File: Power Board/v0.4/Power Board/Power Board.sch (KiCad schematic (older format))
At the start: 31 parts, among them J1 Battery In, J2 JST B2PS-VH, J3 JST B2PS-VH, J4 JST B2PS-VH, J5 JST B2PS-VH, J6 JST B2PS-VH, J7 JST B2PS-VH, J8 Molex 70553-0006, J9 Conn_02x05_Odd_Even, SW1 SW_Push

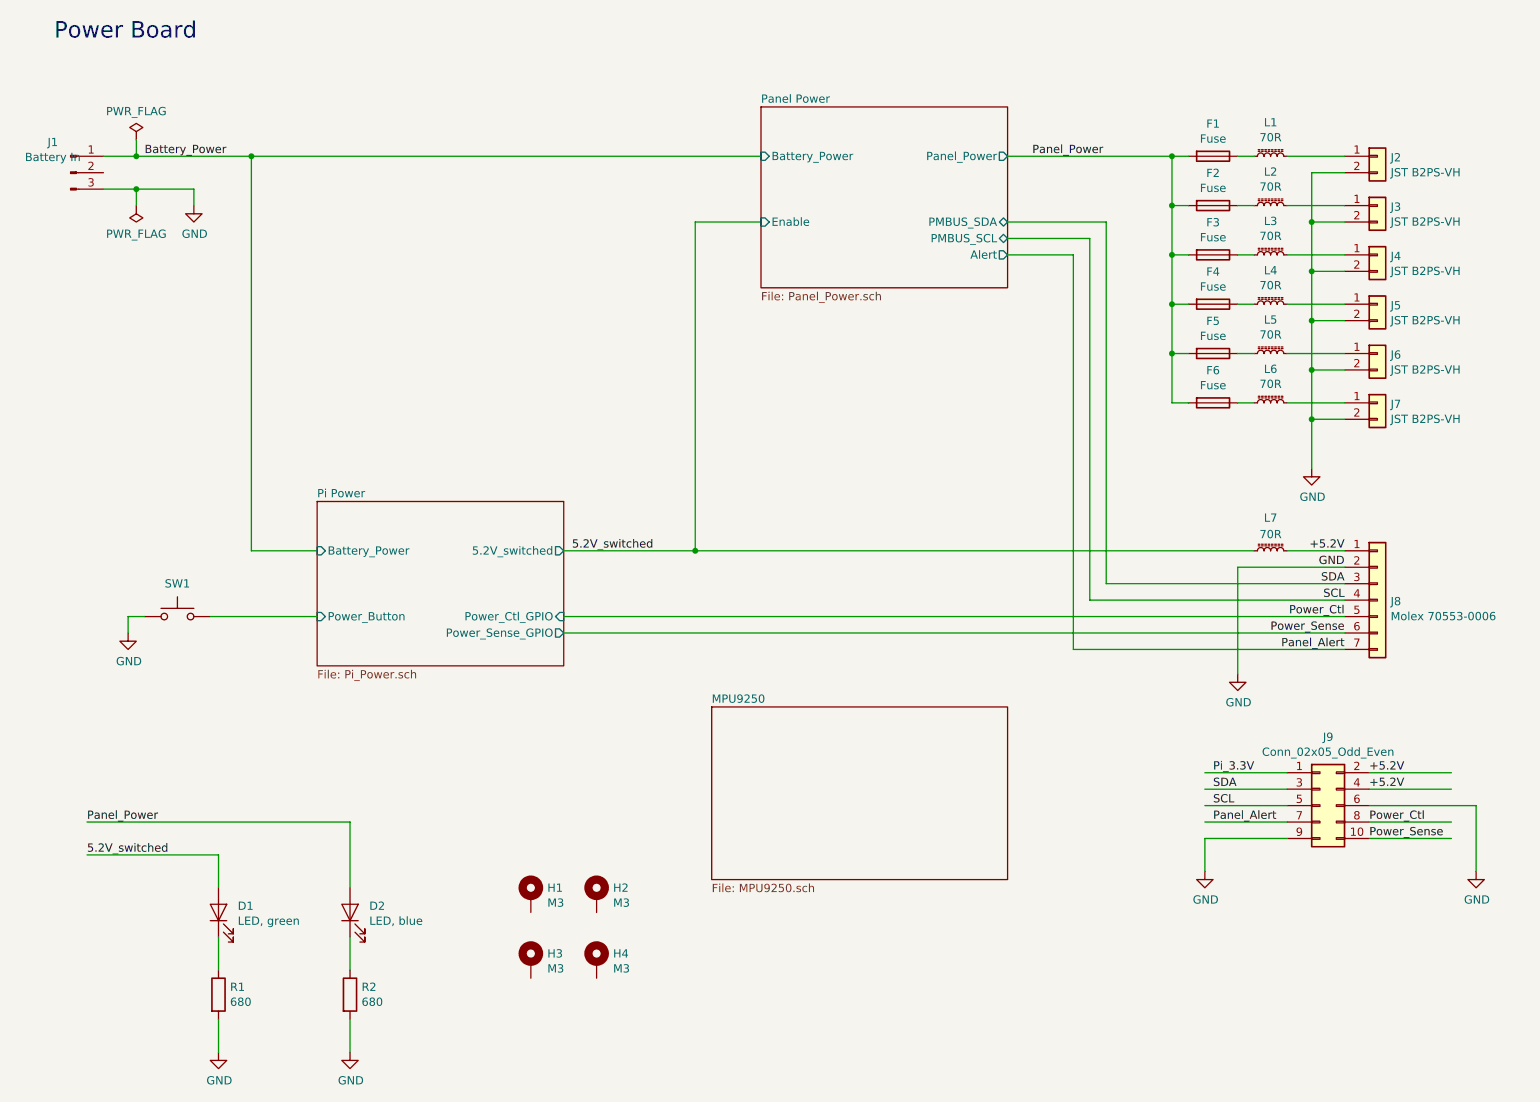
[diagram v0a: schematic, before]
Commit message: Updated board dimensions and mt. holes, tweaked MPU schematic.
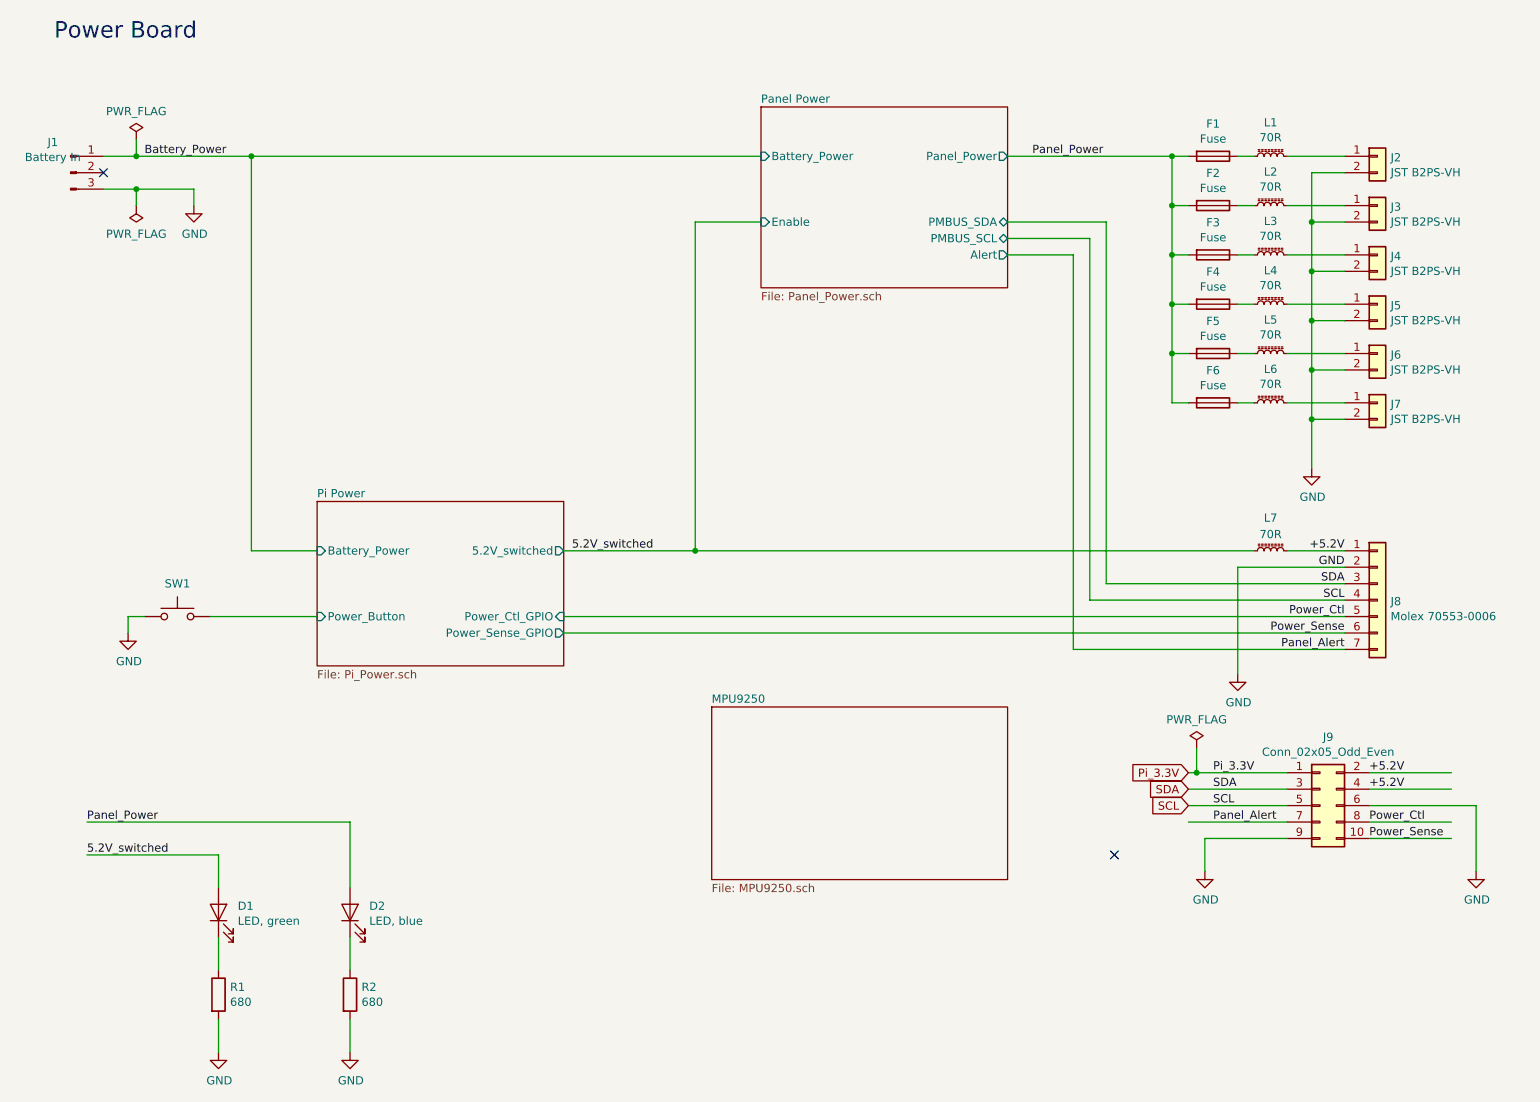
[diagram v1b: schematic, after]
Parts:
- removed H1, H2, H3, H4: M3, MountingHole:MountingHole_3.2mm_M3_Pad_Via, symbol Mechanical:MountingHole_Pad
- J9: footprint Connector_PinHeader_2.54mm:PinHeader_2x05_P2.54mm_Vertical -> Connector_JST:JST_PUD_S10B-PUDSS-1_2x05_P2.00mm_Horizontal
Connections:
- wire segments 87 -> 89
- no-connect marks 0 -> 2
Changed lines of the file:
@@
-$EndComp
-$Comp
-L Mechanical:MountingHole_Pad H1
-U 1 1 5CADB5EA
-P 3900 6400
-F 0 "H1" H 4000 6449 50  0000 L CNN
-F 1 "M3" H 4000 6358 50  0000 L CNN
-F 2 "MountingHole:MountingHole_3.2mm_M3_Pad_Via" H 3900 6400 50  0001 C CNN
-F 3 "~" H 3900 6400 50  0001 C CNN
-F 4 "-" H 0   0   50  0001 C CNN "Digikey No."
-F 5 "-" H 0   0   50  0001 C CNN "Manufacturer"
-F 6 "-" H 0   0   50  0001 C CNN "Part No."
-	1    3900 6400
-	1    0    0    -1
-$EndComp
-$Comp
-L Mechanical:MountingHole_Pad H2
-U 1 1 5CADBAB3
-P 4300 6400
-F 0 "H2" H 4400 6449 50  0000 L CNN
-F 1 "M3" H 4400 6358 50  0000 L CNN
-F 2 "MountingHole:MountingHole_3.2mm_M3_Pad_Via" H 4300 6400 50  0001 C CNN
-F 3 "~" H 4300 6400 50  0001 C CNN
-F 4 "-" H 0   0   50  0001 C CNN "Digikey No."
-F 5 "-" H 0   0   50  0001 C CNN "Manufacturer"
-F 6 "-" H 0   0   50  0001 C CNN "Part No."
-	1    4300 6400
-	1    0    0    -1
-$EndComp
-$Comp
-L Mechanical:MountingHole_Pad H4
-U 1 1 5CADBCBF
-P 4300 6800
-F 0 "H4" H 4400 6849 50  0000 L CNN
-F 1 "M3" H 4400 6758 50  0000 L CNN
-F 2 "MountingHole:MountingHole_3.2mm_M3_Pad_Via" H 4300 6800 50  0001 C CNN
-F 3 "~" H 4300 6800 50  0001 C CNN
-F 4 "-" H 0   0   50  0001 C CNN "Digikey No."
-F 5 "-" H 0   0   50  0001 C CNN "Manufacturer"
-F 6 "-" H 0   0   50  0001 C CNN "Part No."
-	1    4300 6800
-	1    0    0    -1
-$EndComp
-$Comp
-L Mechanical:MountingHole_Pad H3
-U 1 1 5CADBD88
-P 3900 6800
-F 0 "H3" H 4000 6849 50  0000 L CNN
-F 1 "M3" H 4000 6758 50  0000 L CNN
-F 2 "MountingHole:MountingHole_3.2mm_M3_Pad_Via" H 3900 6800 50  0001 C CNN
-F 3 "~" H 3900 6800 50  0001 C CNN
-F 4 "-" H 0   0   50  0001 C CNN "Digikey No."
-F 5 "-" H 0   0   50  0001 C CNN "Manufacturer"
-F 6 "-" H 0   0   50  0001 C CNN "Part No."
-	1    3900 6800
-	1    0    0    -1
 $EndComp
 $Comp
@@
 F 0 "J9" H 8750 6267 50  0000 C CNN
 F 1 "Conn_02x05_Odd_Even" H 8750 6176 50  0000 C CNN
-F 2 "Connector_PinHeader_2.54mm:PinHeader_2x05_P2.54mm_Vertical" H 8700 5850 50  0001 C CNN
+F 2 "Connector_JST:JST_PUD_S10B-PUDSS-1_2x05_P2.00mm_Horizontal" H 8700 5850 50  0001 C CNN
 F 3 "~" H 8700 5850 50  0001 C CNN
 	1    8700 5850
@@
 	9000 5850 9650 5850
 Wire Wire Line
-	8000 5650 8500 5650
+	7900 5750 8500 5750
 Wire Wire Line
-	8000 5750 8500 5750
+	7900 5850 8500 5850
 Wire Wire Line
-	8000 5850 8500 5850
-Wire Wire Line
-	8000 5950 8500 5950
+	7900 5950 8500 5950
 Wire Wire Line
 	8000 6050 8500 6050
@@
 	8000 6050 8000 6250
 $Comp
-L power:GND #PWR?
+L power:GND #PWR0109
 U 1 1 5CC03CFB
 P 8000 6250
-F 0 "#PWR?" H 8000 6000 50  0001 C CNN
+F 0 "#PWR0109" H 8000 6000 50  0001 C CNN
 F 1 "GND" H 8005 6077 50  0000 C CNN
 F 2 "" H 8000 6250 50  0001 C CNN
@@
 $EndComp
 $Comp
-L power:GND #PWR?
+L power:GND #PWR0110
 U 1 1 5CC046D5
 P 9650 6250
-F 0 "#PWR?" H 9650 6000 50  0001 C CNN
+F 0 "#PWR0110" H 9650 6000 50  0001 C CNN
 F 1 "GND" H 9655 6077 50  0000 C CNN
 F 2 "" H 9650 6250 50  0001 C CNN
@@
 	1    0    0    -1
 $EndComp
+NoConn ~ 1300 2000
+NoConn ~ 7450 6150
+Text GLabel 7900 5650 0    50   Input ~ 0
+Pi_3.3V
+Text GLabel 7900 5750 0    50   Input ~ 0
+SDA
+Text GLabel 7900 5850 0    50   Input ~ 0
+SCL
+$Comp
+L power:PWR_FLAG #FLG0101
+U 1 1 5CB3FC6A
+P 7950 5500
+F 0 "#FLG0101" H 7950 5575 50  0001 C CNN
+F 1 "PWR_FLAG" H 7950 5673 50  0000 C CNN
+F 2 "" H 7950 5500 50  0001 C CNN
+F 3 "~" H 7950 5500 50  0001 C CNN
+	1    7950 5500
+	1    0    0    -1
+$EndComp
+Wire Wire Line
+	7950 5500 7950 5650
+Wire Wire Line
+	7900 5650 7950 5650
+Connection ~ 7950 5650
+Wire Wire Line
+	7950 5650 8500 5650
 $EndSCHEMATC

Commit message: Revert "Updated board dimensions and mt. holes, tweaked MPU schematic."
This reverts commit 6936a160ef8a0f8efd2e8f2d18775030a6ae8800.
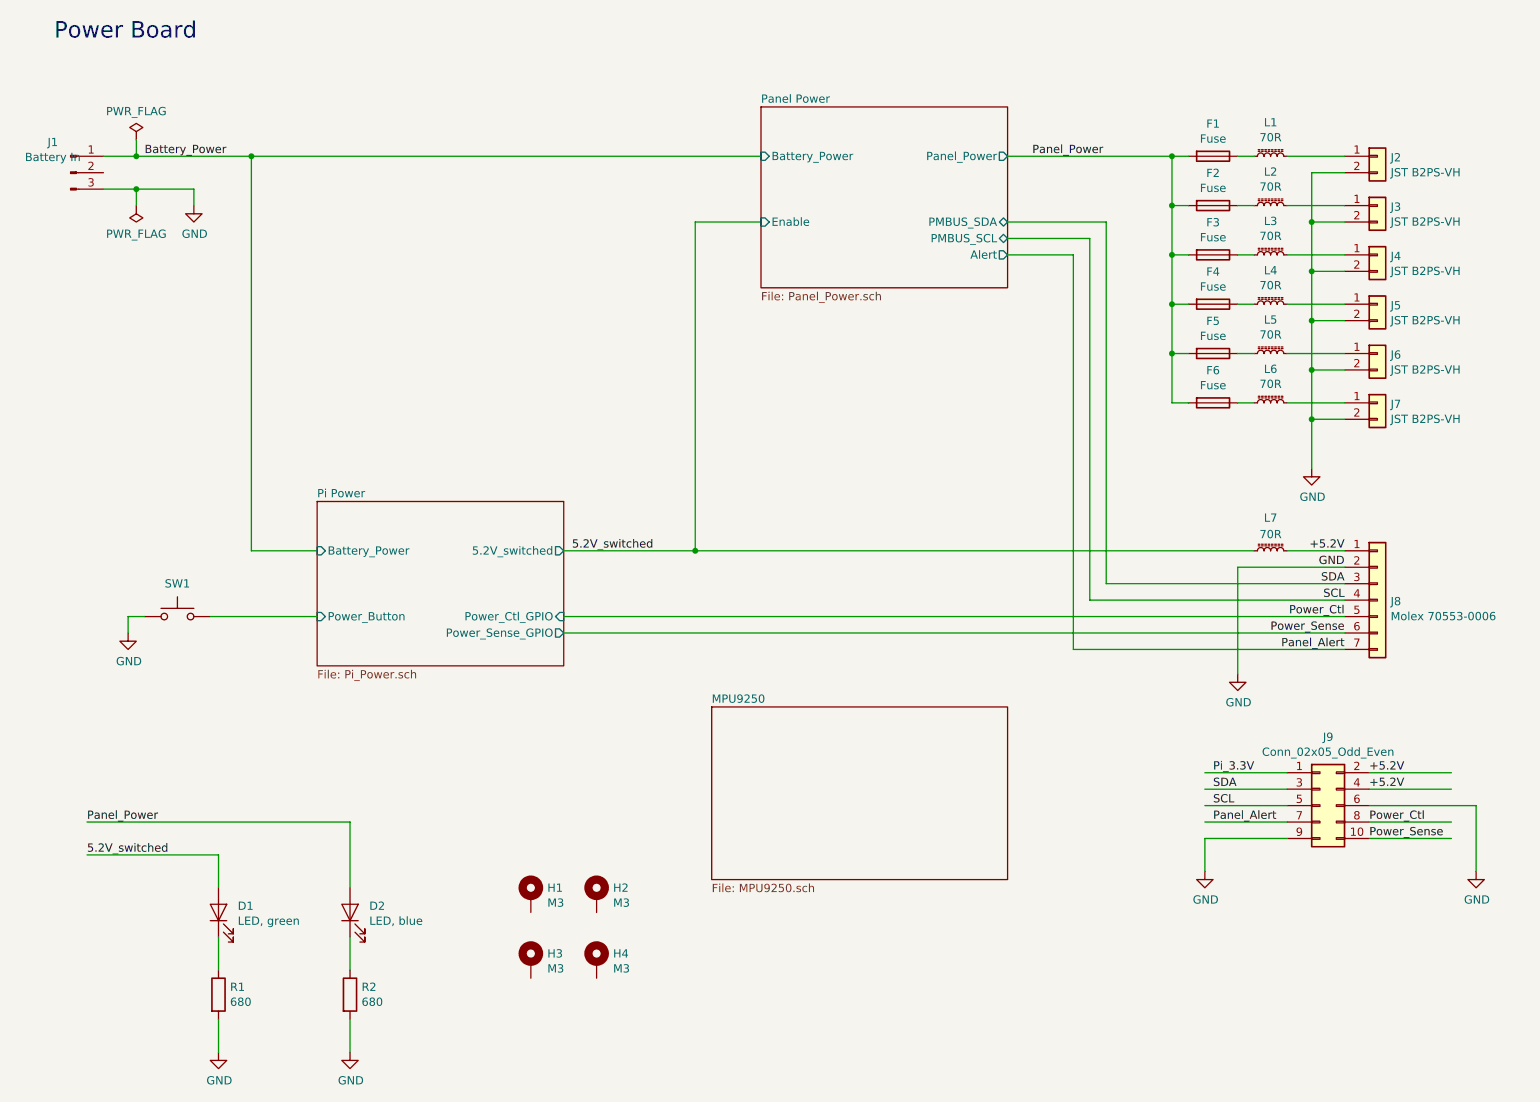
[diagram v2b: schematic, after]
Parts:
- added H1, H2, H3, H4: M3, MountingHole:MountingHole_3.2mm_M3_Pad_Via, symbol Mechanical:MountingHole_Pad
- J9: footprint Connector_JST:JST_PUD_S10B-PUDSS-1_2x05_P2.00mm_Horizontal -> Connector_PinHeader_2.54mm:PinHeader_2x05_P2.54mm_Vertical
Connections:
- wire segments 89 -> 87
- no-connect marks 2 -> 0
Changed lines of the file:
@@
+$EndComp
+$Comp
+L Mechanical:MountingHole_Pad H1
+U 1 1 5CADB5EA
+P 3900 6400
+F 0 "H1" H 4000 6449 50  0000 L CNN
+F 1 "M3" H 4000 6358 50  0000 L CNN
+F 2 "MountingHole:MountingHole_3.2mm_M3_Pad_Via" H 3900 6400 50  0001 C CNN
+F 3 "~" H 3900 6400 50  0001 C CNN
+F 4 "-" H 0   0   50  0001 C CNN "Digikey No."
+F 5 "-" H 0   0   50  0001 C CNN "Manufacturer"
+F 6 "-" H 0   0   50  0001 C CNN "Part No."
+	1    3900 6400
+	1    0    0    -1
+$EndComp
+$Comp
+L Mechanical:MountingHole_Pad H2
+U 1 1 5CADBAB3
+P 4300 6400
+F 0 "H2" H 4400 6449 50  0000 L CNN
+F 1 "M3" H 4400 6358 50  0000 L CNN
+F 2 "MountingHole:MountingHole_3.2mm_M3_Pad_Via" H 4300 6400 50  0001 C CNN
+F 3 "~" H 4300 6400 50  0001 C CNN
+F 4 "-" H 0   0   50  0001 C CNN "Digikey No."
+F 5 "-" H 0   0   50  0001 C CNN "Manufacturer"
+F 6 "-" H 0   0   50  0001 C CNN "Part No."
+	1    4300 6400
+	1    0    0    -1
+$EndComp
+$Comp
+L Mechanical:MountingHole_Pad H4
+U 1 1 5CADBCBF
+P 4300 6800
+F 0 "H4" H 4400 6849 50  0000 L CNN
+F 1 "M3" H 4400 6758 50  0000 L CNN
+F 2 "MountingHole:MountingHole_3.2mm_M3_Pad_Via" H 4300 6800 50  0001 C CNN
+F 3 "~" H 4300 6800 50  0001 C CNN
+F 4 "-" H 0   0   50  0001 C CNN "Digikey No."
+F 5 "-" H 0   0   50  0001 C CNN "Manufacturer"
+F 6 "-" H 0   0   50  0001 C CNN "Part No."
+	1    4300 6800
+	1    0    0    -1
+$EndComp
+$Comp
+L Mechanical:MountingHole_Pad H3
+U 1 1 5CADBD88
+P 3900 6800
+F 0 "H3" H 4000 6849 50  0000 L CNN
+F 1 "M3" H 4000 6758 50  0000 L CNN
+F 2 "MountingHole:MountingHole_3.2mm_M3_Pad_Via" H 3900 6800 50  0001 C CNN
+F 3 "~" H 3900 6800 50  0001 C CNN
+F 4 "-" H 0   0   50  0001 C CNN "Digikey No."
+F 5 "-" H 0   0   50  0001 C CNN "Manufacturer"
+F 6 "-" H 0   0   50  0001 C CNN "Part No."
+	1    3900 6800
+	1    0    0    -1
 $EndComp
 $Comp
@@
 F 0 "J9" H 8750 6267 50  0000 C CNN
 F 1 "Conn_02x05_Odd_Even" H 8750 6176 50  0000 C CNN
-F 2 "Connector_JST:JST_PUD_S10B-PUDSS-1_2x05_P2.00mm_Horizontal" H 8700 5850 50  0001 C CNN
+F 2 "Connector_PinHeader_2.54mm:PinHeader_2x05_P2.54mm_Vertical" H 8700 5850 50  0001 C CNN
 F 3 "~" H 8700 5850 50  0001 C CNN
 	1    8700 5850
@@
 	9000 5850 9650 5850
 Wire Wire Line
-	7900 5750 8500 5750
+	8000 5650 8500 5650
 Wire Wire Line
-	7900 5850 8500 5850
+	8000 5750 8500 5750
 Wire Wire Line
-	7900 5950 8500 5950
+	8000 5850 8500 5850
+Wire Wire Line
+	8000 5950 8500 5950
 Wire Wire Line
 	8000 6050 8500 6050
@@
 	8000 6050 8000 6250
 $Comp
-L power:GND #PWR0109
+L power:GND #PWR?
 U 1 1 5CC03CFB
 P 8000 6250
-F 0 "#PWR0109" H 8000 6000 50  0001 C CNN
+F 0 "#PWR?" H 8000 6000 50  0001 C CNN
 F 1 "GND" H 8005 6077 50  0000 C CNN
 F 2 "" H 8000 6250 50  0001 C CNN
@@
 $EndComp
 $Comp
-L power:GND #PWR0110
+L power:GND #PWR?
 U 1 1 5CC046D5
 P 9650 6250
-F 0 "#PWR0110" H 9650 6000 50  0001 C CNN
+F 0 "#PWR?" H 9650 6000 50  0001 C CNN
 F 1 "GND" H 9655 6077 50  0000 C CNN
 F 2 "" H 9650 6250 50  0001 C CNN
@@
 	1    0    0    -1
 $EndComp
-NoConn ~ 1300 2000
-NoConn ~ 7450 6150
-Text GLabel 7900 5650 0    50   Input ~ 0
-Pi_3.3V
-Text GLabel 7900 5750 0    50   Input ~ 0
-SDA
-Text GLabel 7900 5850 0    50   Input ~ 0
-SCL
-$Comp
-L power:PWR_FLAG #FLG0101
-U 1 1 5CB3FC6A
-P 7950 5500
-F 0 "#FLG0101" H 7950 5575 50  0001 C CNN
-F 1 "PWR_FLAG" H 7950 5673 50  0000 C CNN
-F 2 "" H 7950 5500 50  0001 C CNN
-F 3 "~" H 7950 5500 50  0001 C CNN
-	1    7950 5500
-	1    0    0    -1
-$EndComp
-Wire Wire Line
-	7950 5500 7950 5650
-Wire Wire Line
-	7900 5650 7950 5650
-Connection ~ 7950 5650
-Wire Wire Line
-	7950 5650 8500 5650
 $EndSCHEMATC
